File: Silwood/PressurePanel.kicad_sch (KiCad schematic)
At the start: 10 parts

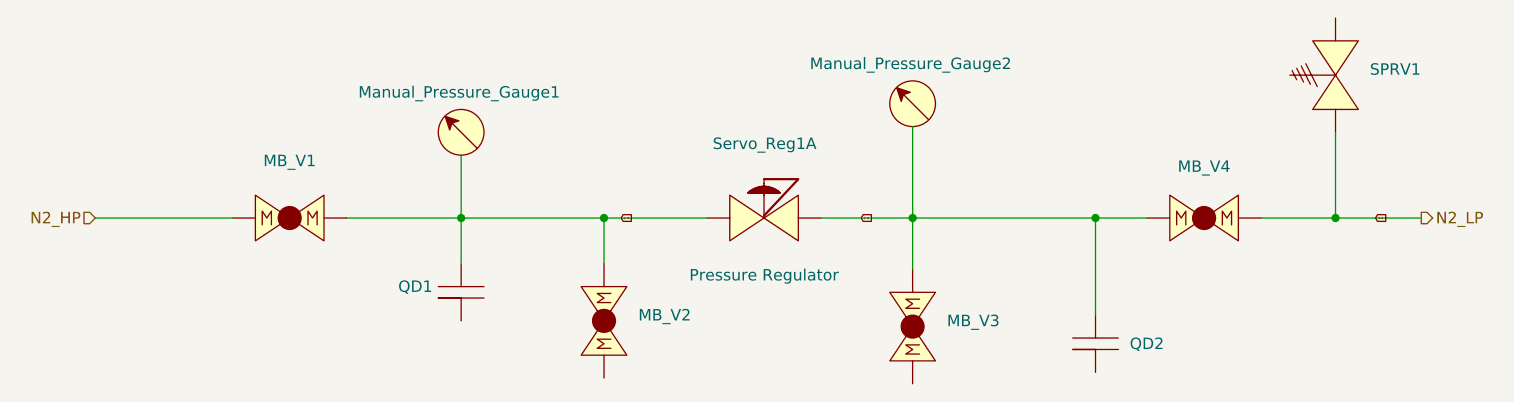
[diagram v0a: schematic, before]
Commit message: Formatiing
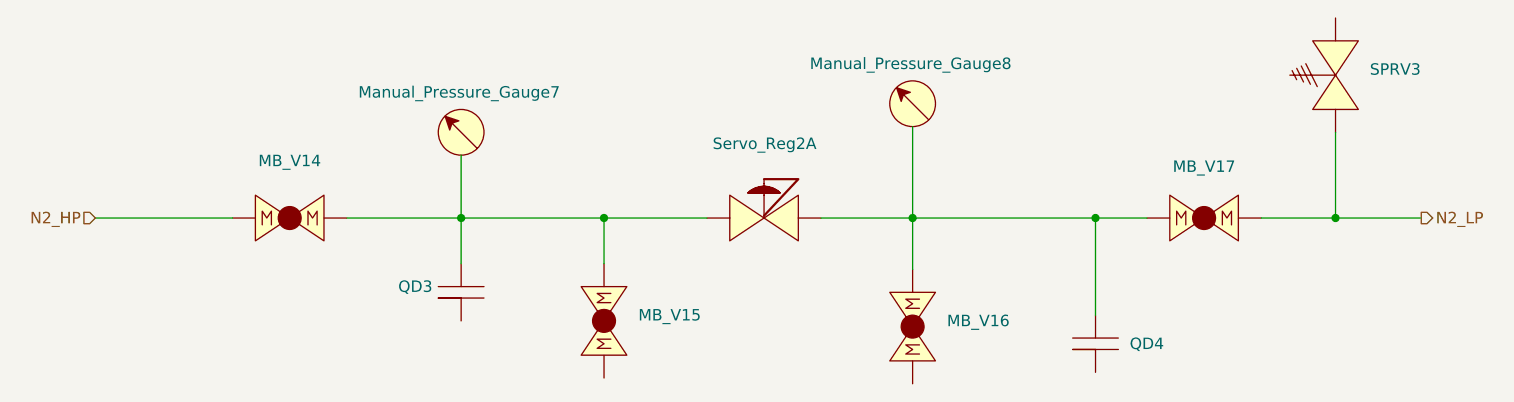
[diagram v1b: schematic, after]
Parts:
- renumbered MB_V1 to MB_V14, MB_V2 to MB_V15, MB_V3 to MB_V16, MB_V4 to MB_V17, Manual_Pressure_Gauge1 to Manual_Pressure_Gauge7, Manual_Pressure_Gauge2 to Manual_Pressure_Gauge8, QD1 to QD3, QD2 to QD4, SPRV1 to SPRV3, Servo_Reg1 to Servo_Reg2
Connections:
- net 3-8 is gone; now on net N2_LP: MB_V17., SPRV3.
- net at QD4.: now also MB_V16., MB_V17., Manual_Pressure_Gauge8., Servo_Reg2.
- net N2_LP: now reaches SPRV3.
- removed net 1-4: MB_V14., MB_V15., MB_V16., MB_V17., Manual_Pressure_Gauge7., Manual_Pressure_Gauge8., QD3., QD4., Servo_Reg2.
- new net: MB_V14., MB_V15., Manual_Pressure_Gauge7., QD3., Servo_Reg2.
